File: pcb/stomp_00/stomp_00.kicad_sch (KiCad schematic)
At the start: 13 parts, among them J1 Conn_01x18_Pin, J10 Conn_01x18_Pin, J2 Conn_01x18_Pin, J3 Conn_01x18_Pin, J4 Conn_01x18_Pin, J5 Conn_01x18_Pin, J6 Conn_01x18_Pin, J7 Conn_01x18_Pin, J8 Conn_01x18_Pin, J9 Conn_01x18_Pin, U1 Teensy4.1

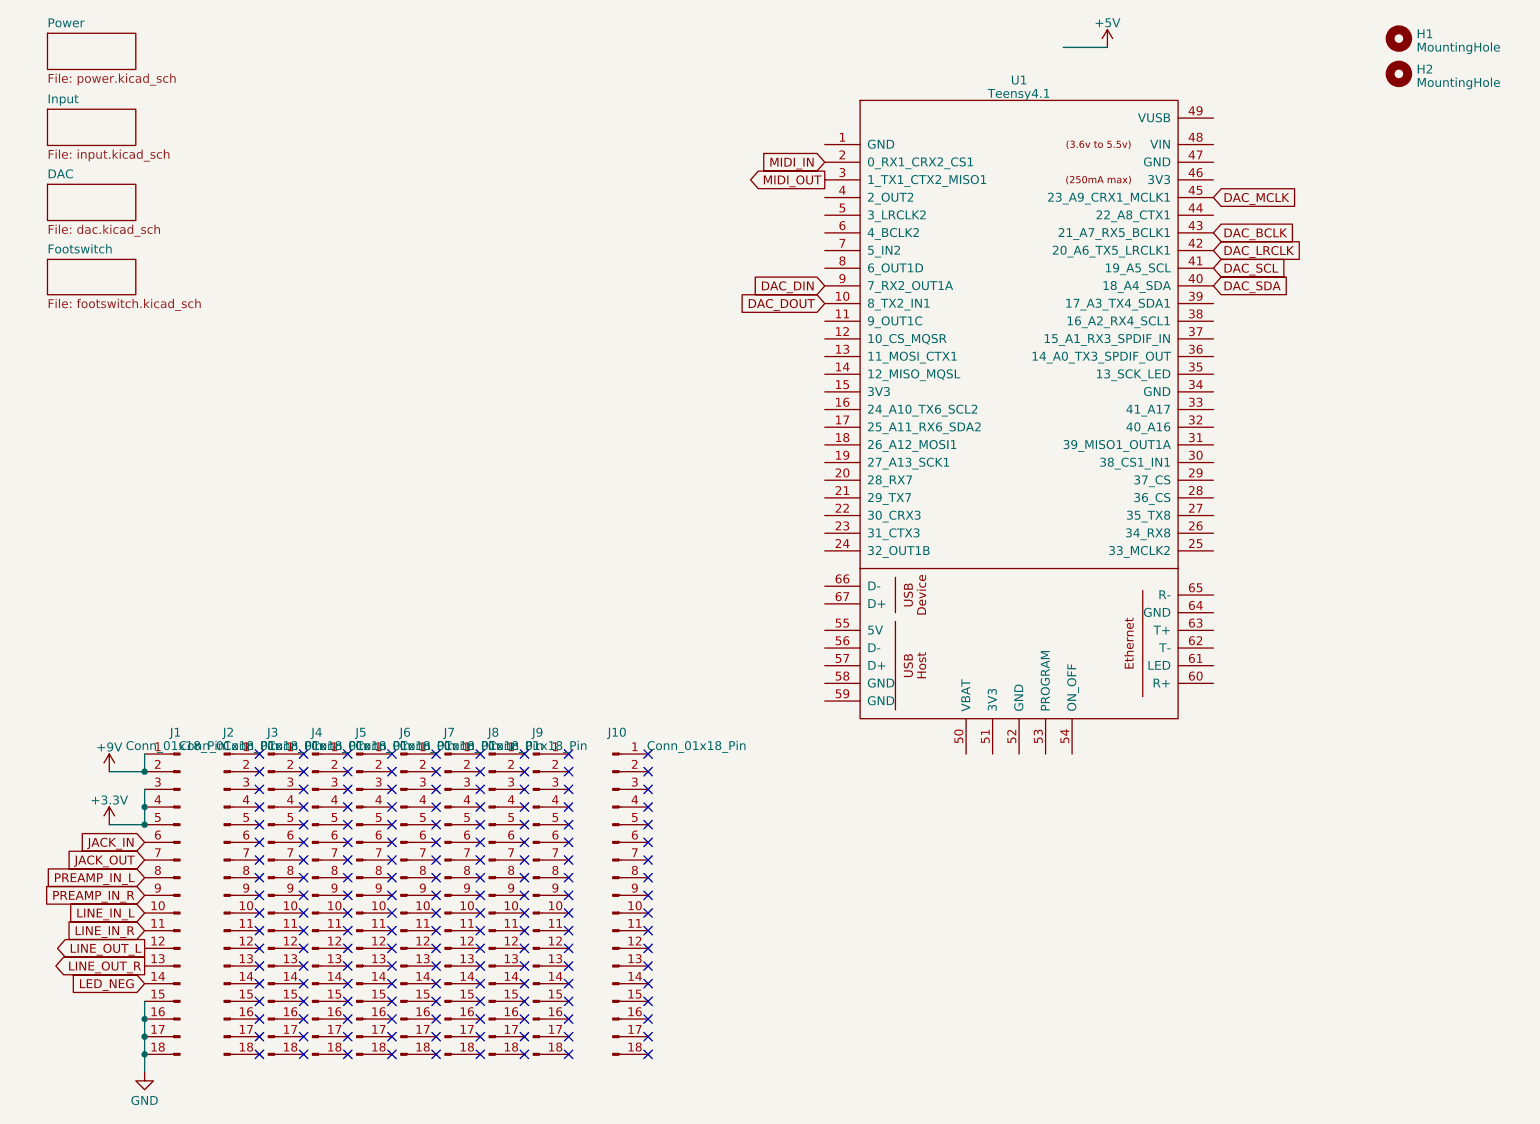
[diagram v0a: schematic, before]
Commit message: fixing ERC stuff, importing PCB into freecad
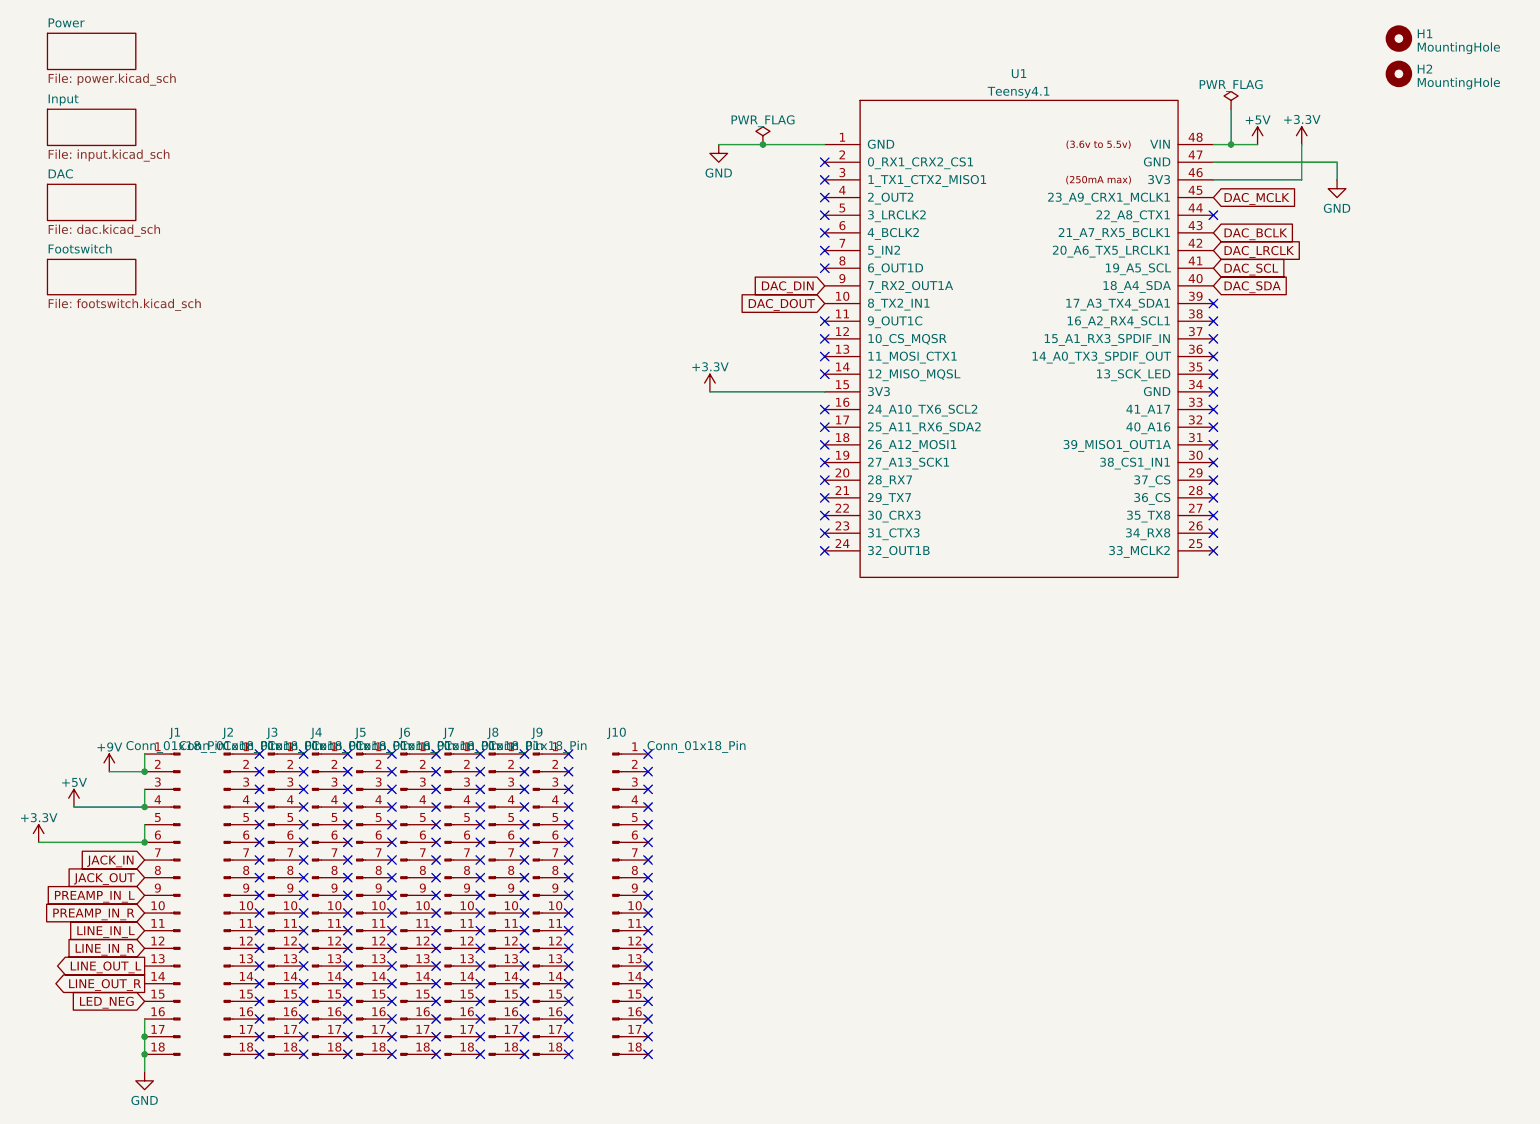
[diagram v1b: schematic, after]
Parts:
- U1: symbol teensy:Teensy4.1 -> stomp:Teensy4.1_simplified
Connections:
- net +3.3V: now also J1.6 (Pin_6), U1.15 (3V3), U1.46 (3V3); no longer J1.3 (Pin_3), J1.4 (Pin_4)
- net +5V: now also J1.3 (Pin_3), J1.4 (Pin_4), U1.48 (VIN)
- net GND: now also U1.1 (GND), U1.47 (GND); no longer J1.15 (Pin_15)
- net JACK_IN: now also J1.7 (Pin_7); no longer J1.6 (Pin_6)
- net JACK_OUT: now also J1.8 (Pin_8); no longer J1.7 (Pin_7)
- net LED_NEG: now also J1.15 (Pin_15); no longer J1.14 (Pin_14)
- net LINE_IN_L: now also J1.11 (Pin_11); no longer J1.10 (Pin_10)
- net LINE_IN_R: now also J1.12 (Pin_12); no longer J1.11 (Pin_11)
- net LINE_OUT_L: now also J1.13 (Pin_13); no longer J1.12 (Pin_12)
- net LINE_OUT_R: now also J1.14 (Pin_14); no longer J1.13 (Pin_13)
- net PREAMP_IN_L: now also J1.9 (Pin_9); no longer J1.8 (Pin_8)
- net PREAMP_IN_R: now also J1.10 (Pin_10); no longer J1.9 (Pin_9)
- net MIDI_IN: no longer names the net of U1.2 (0_RX1_CRX2_CS1)
- net MIDI_OUT: no longer names the net of U1.3 (1_TX1_CTX2_MISO1)
- no-connect marks 162 -> 198
